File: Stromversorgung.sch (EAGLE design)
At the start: 17 parts, among them IC1 LM2574N-3.3, X1 MSTBV4, X2 Power ext., 5V 1A, X4 Power int., 5V 3A

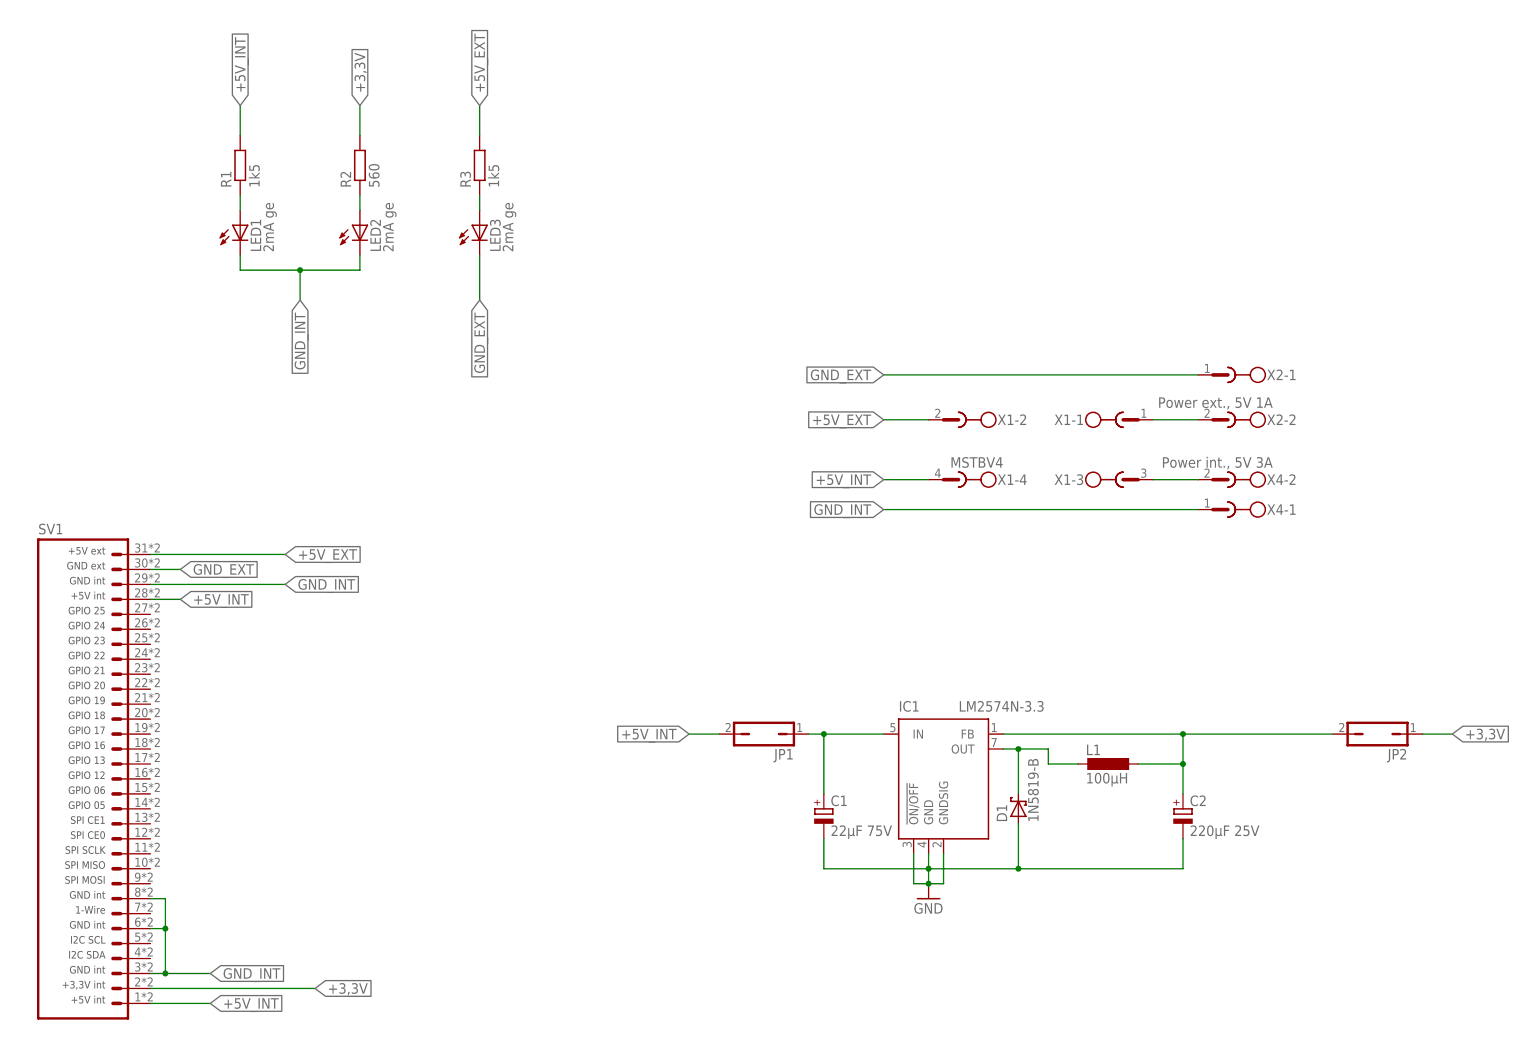
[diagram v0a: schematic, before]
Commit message: Pi und Stromversorgung Rev. 2019
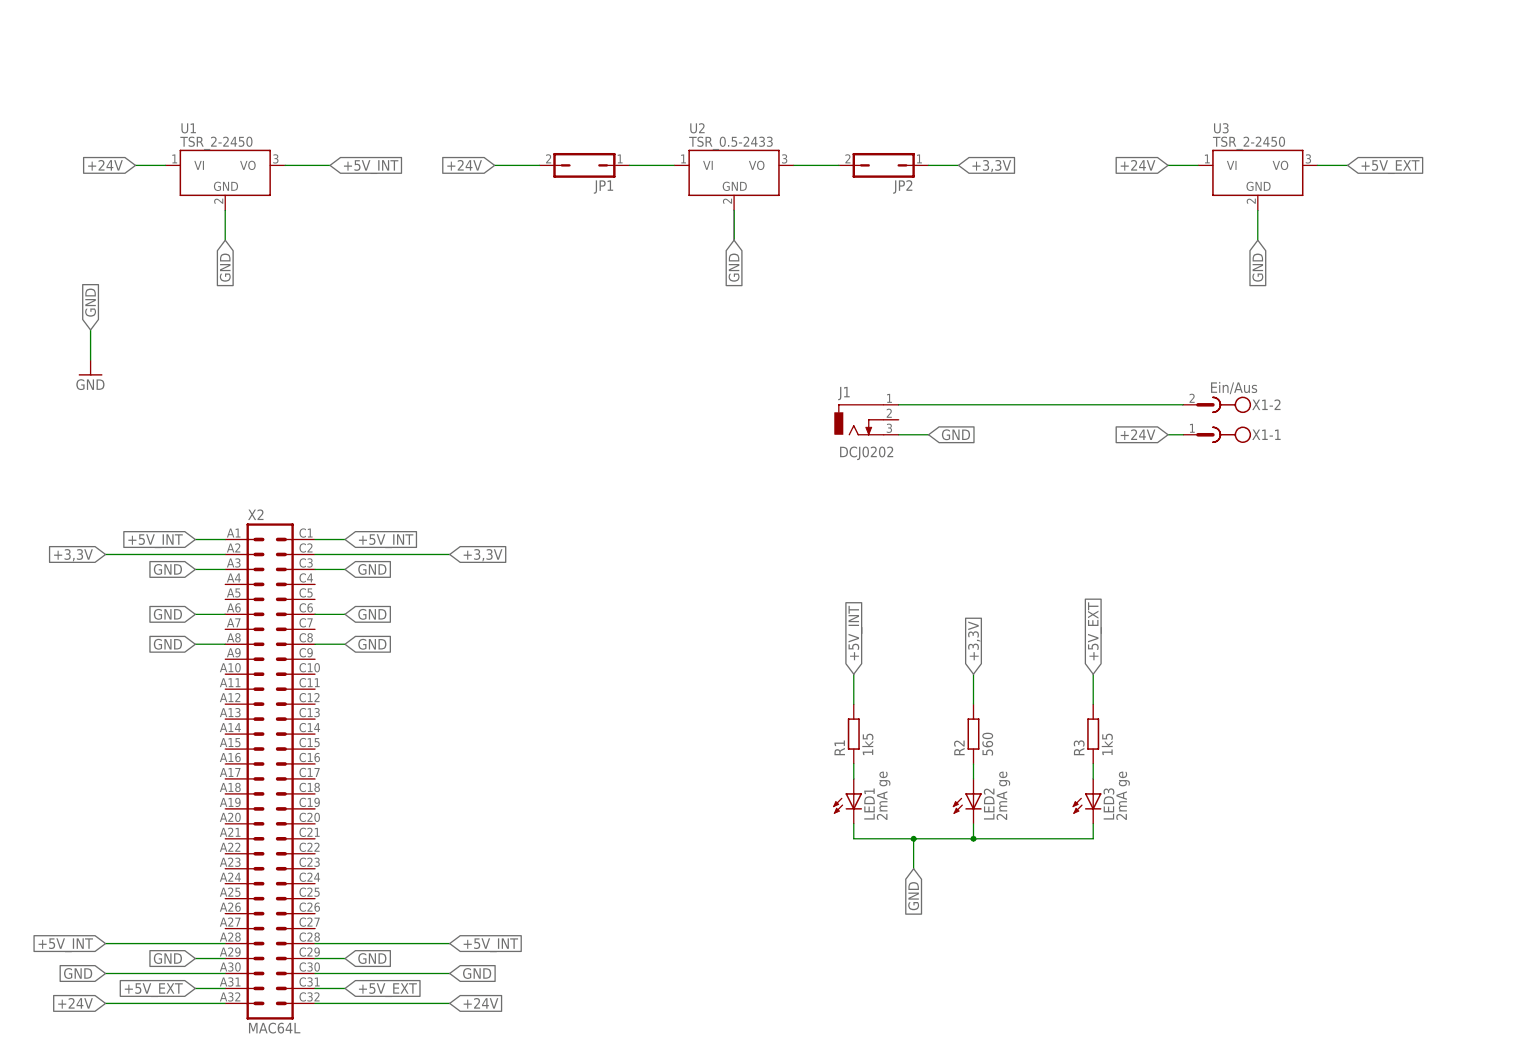
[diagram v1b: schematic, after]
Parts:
- removed C1: 22µF 75V, rcl:CPOL-EUE2.5-5
- removed C2: 220µF 25V, rcl:CPOL-EUE2.5-5
- removed D1: 1N5819-B, diode:1N5819-B
- removed IC1: LM2574N-3.3, linear:LM2574N-3.3
- removed L1: 100µH, rcl:L-EU6000-XXX-RC
- removed SV1: PLATINENVERBINDER-31SMD, homepi:PLATINENVERBINDER-31SMD
- removed X4: Power int., 5V 3A, con-phoenix-508:MSTBV2
- added J1: DCJ0202, con-jack:DCJ0202
- added U1, U3: TSR_2-2450, _traco_tsr-1:TSR_1-2450
- added U2: TSR_0.5-2433, _traco_tsr-1:TSR_1-2433
- X1: value MSTBV4 -> Ein/Aus; device con-phoenix-508:MSTBV4 -> con-phoenix-508:MSTBV2
- X2: value Power ext., 5V 1A -> MAC64L; device con-phoenix-508:MSTBV2 -> con-vg:MAC64L
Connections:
- removed net +3,3V_INT_1: C2.+, IC1.FB, JP2.2, L1.1
- removed net GND_EXT: LED3.C, SV1.30, X2-1.1
- removed net GND_INT: C1.-, C2.-, D1.A, IC1.!ON/OFF, IC1.GND@PWR, IC1.GNDSIG, LED1.C, LED2.C, SV1.29, SV1.3, SV1.6, SV1.8, X4-1.1
- removed net LM2574_IN: C1.+, IC1.IN, JP1.1
- removed net LM2574_OUT: D1.C, IC1.OUT, L1.2
- removed net N$3: X1-3.1, X4-2.1
- new net +24V: JP1.2, U1.VI, U3.VI, X1-1.1, X2.A32, X2.C32
- new net GND: J1.3, LED1.C, LED2.C, LED3.C, U1.GND, U2.GND, U3.GND, X2.A29, X2.A3, X2.A30, X2.A6, X2.A8, X2.C29, X2.C3, X2.C30, X2.C6, X2.C8
- new net N$2: JP2.2, U2.VO
- new net VI: JP1.1, U2.VI
- net +3,3V: now also X2.A2, X2.C2; no longer SV1.2
- net +5V_EXT: now also U3.VO, X2.A31, X2.C31; no longer SV1.31, X1-2.1
- net +5V_INT: now also U1.VO, X2.A1, X2.A28, X2.C1, X2.C28; no longer JP1.2, SV1.1, SV1.28, X1-4.1
- net N$1: now also J1.1, X1-2.1; no longer X1-1.1, X2-2.1
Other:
- moved on the sheet: JP1, JP2, LED1, LED2, LED3, R1, R2, R3, X1-1, X1-2
